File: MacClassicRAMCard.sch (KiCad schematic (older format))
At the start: 19 parts, among them J1 RAM Exp., U1 AS4C1M16F5, U2 AS4C1M16F5, U3 74LS08

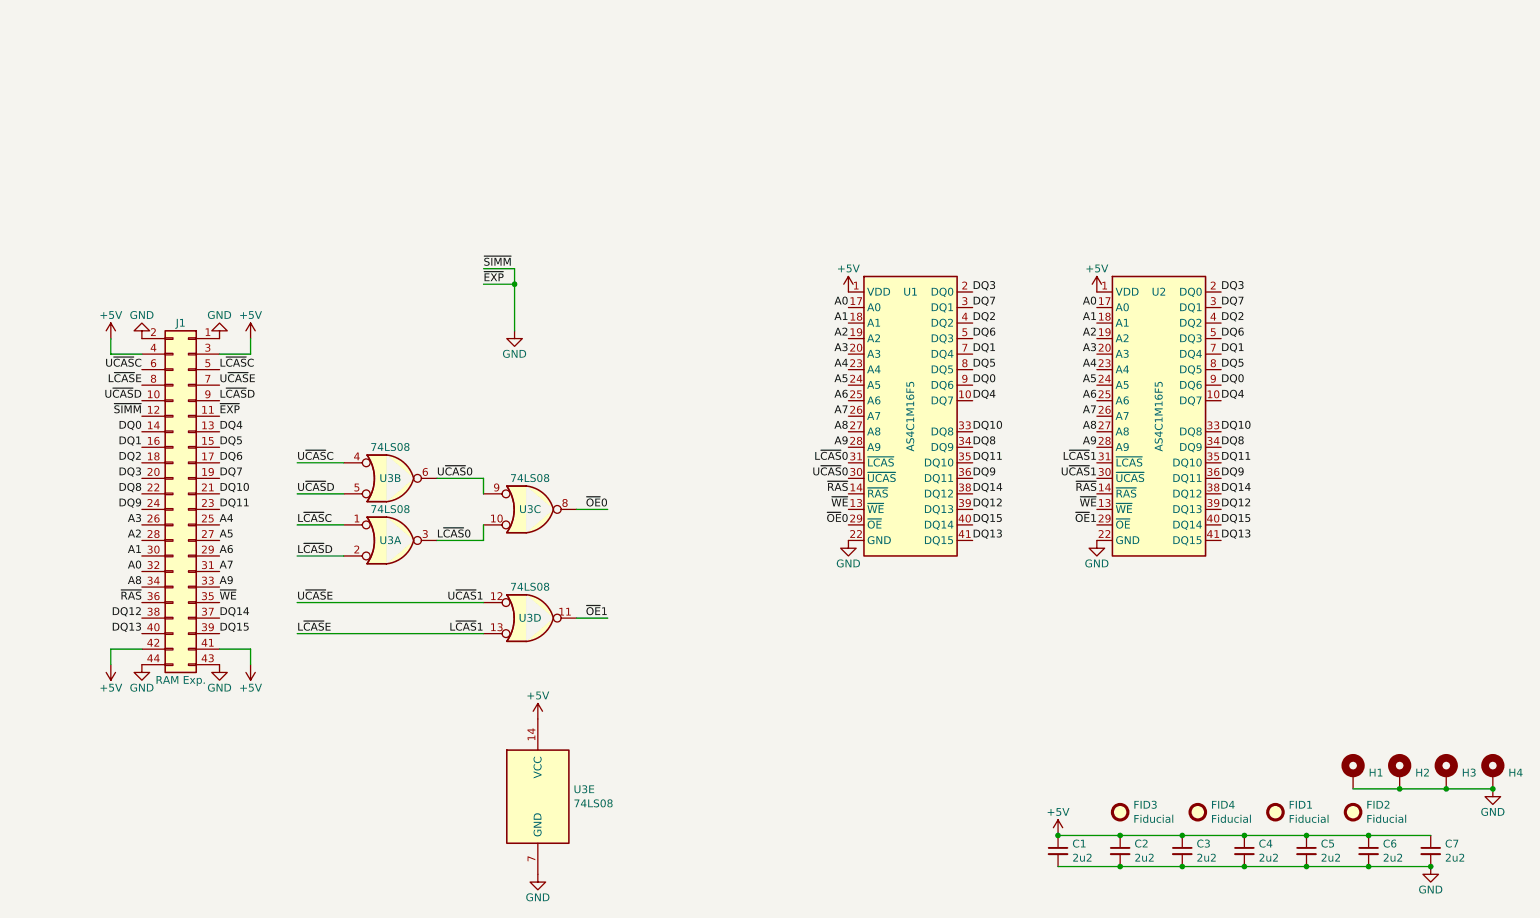
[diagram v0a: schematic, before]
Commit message: As sent to JLC
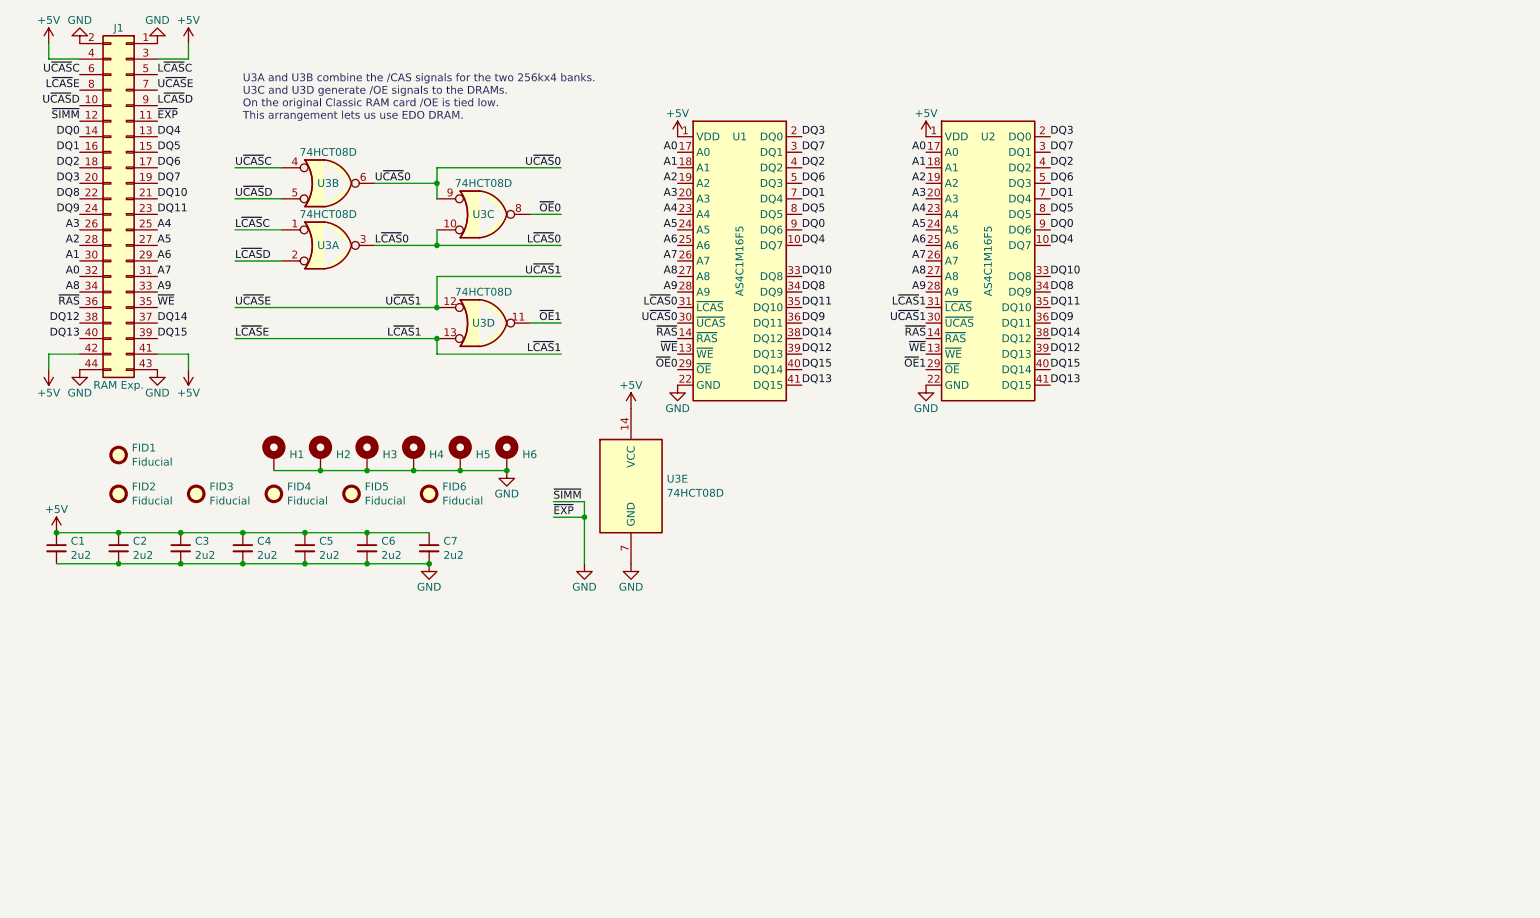
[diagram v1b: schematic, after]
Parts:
- added FID5, FID6: Fiducial, stdpads:Fiducial, symbol Mechanical:Fiducial
- added H5, H6: (no value), stdpads:PasteHole_1.1mm_PTH, symbol Mechanical:MountingHole_Pad
- J1: footprint Connector_PinSocket_2.54mm:PinSocket_2x22_P2.54mm_Horizontal -> stdpads:PinSocket_2x22_P2.54mm_Horizontal
- U3: value 74LS08 -> 74HCT08D
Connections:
- net GND: now also H5.1, H6.1
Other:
- note added: "U3A and U3B combine the /CAS signals for the two 256kx4 banks.\nU3C and U3D generate /OE signals to the DRAMs.\nOn the original Classic RAM card /OE is tied low.\nThis arrangement lets us use EDO DRAM."
- moved on the sheet: C1, C2, C3, C4, C5, C6, C7, FID1, FID2, FID3, FID4, H1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
